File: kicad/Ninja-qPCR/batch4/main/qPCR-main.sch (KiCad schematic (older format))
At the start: 38 parts, among them J1 Raspberry_Pi_3A_Plus_wpi, J2 Conn_01x03_Male, J3 Conn_01x01_Male, J4 Conn_01x01_Male, J5 Conn_02x03_Odd_Even, J6 Conn_02x03_Odd_Even, J7 Conn_02x03_Odd_Even, Q1 Q_NMOS_GSD, Q2 Q_NMOS_GSD, Q3 Q_NMOS_GSD, Q4 Q_NMOS_GSD, Q5 Q_NMOS_GSD, Q6 Q_NMOS_GSD, SW1 TACTILE_4

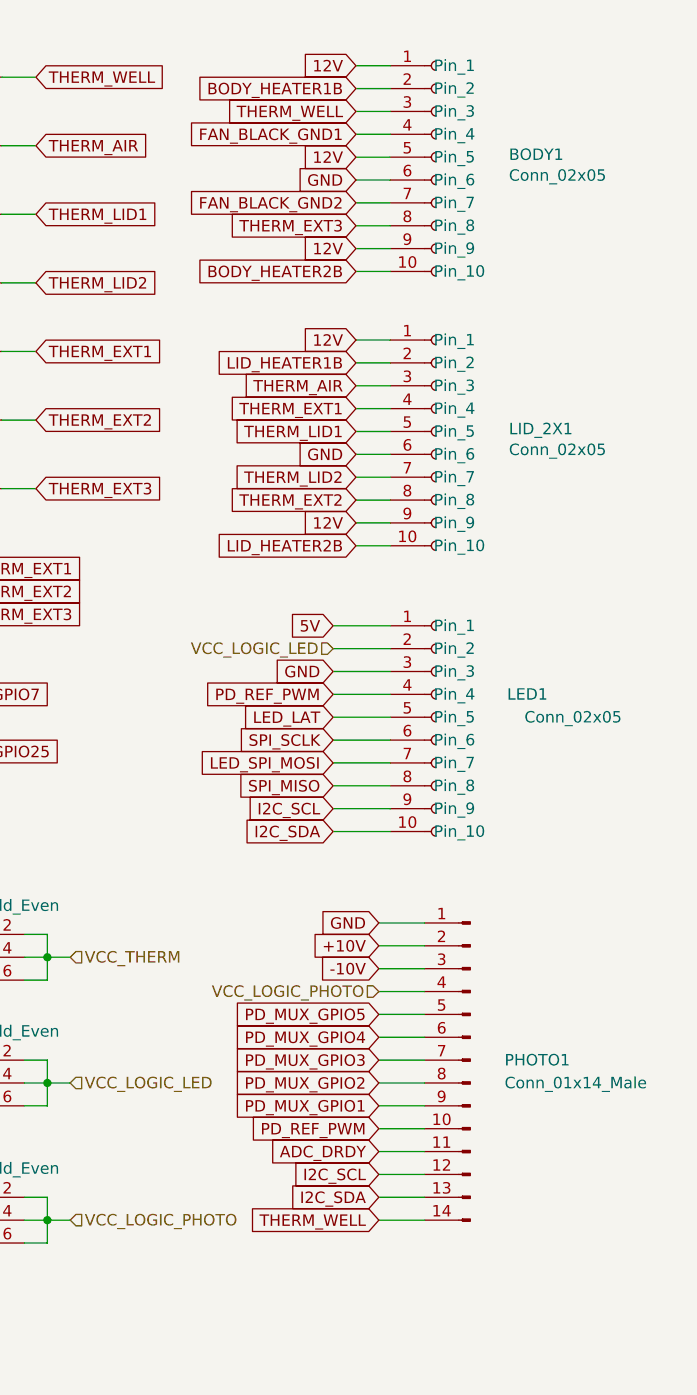
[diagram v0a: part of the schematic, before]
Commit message: add workflow
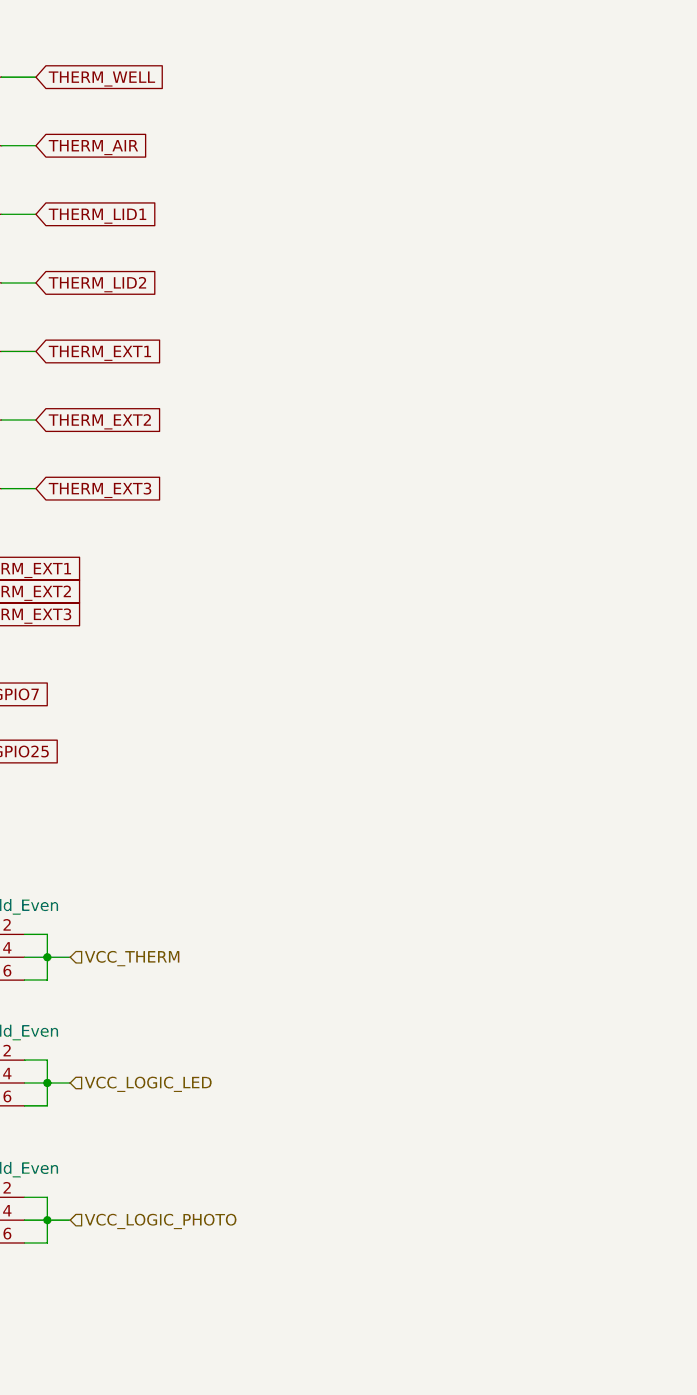
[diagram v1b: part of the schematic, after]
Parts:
- removed BODY1, LED1, LID_2X1: Conn_02x05, Ninja-qPCR:Con_2x05, symbol Ninja-qPCR:Conn_02x05
- removed PHOTO1: Conn_01x14_Male, Pin_Headers:Pin_Header_Straight_1x14_Pitch2.54mm, symbol Connector:Conn_01x14_Male
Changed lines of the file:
@@
 Wire Wire Line
 	2150 2950 2000 2950
-Text GLabel 9950 4700 0    50   Input ~ 0
-GND
-Wire Wire Line
-	9950 4700 10150 4700
-Wire Wire Line
-	10150 4800 9950 4800
-Wire Wire Line
-	9950 4900 10150 4900
-Wire Wire Line
-	10150 5000 9950 5000
-Wire Wire Line
-	9950 5100 10150 5100
-Wire Wire Line
-	10150 5200 9950 5200
-Wire Wire Line
-	9950 5300 10150 5300
-Wire Wire Line
-	10150 5400 9950 5400
-Wire Wire Line
-	9950 5500 10150 5500
-$Comp
-L Ninja-qPCR:Conn_02x05 LED1
-U 1 1 5F7E3B13
-P 10200 3400
-AR Path="/5F7E3B13" Ref="LED1"  Part="1"
-AR Path="/5F708CA1/5F7E3B13" Ref="LED?"  Part="1"
-F 0 "LED1" H 10600 3100 50  0000 C CNN
-F 1 "Conn_02x05" H 10800 3000 50  0000 C CNN
-F 2 "Ninja-qPCR:Con_2x05" H 10000 3500 50  0001 C CNN
-F 3 "" H 10000 3500 50  0001 C CNN
-	1    10200 3400
-	1    0    0    -1
-$EndComp
-Text GLabel 9750 3600 0    50   Input ~ 0
-GND
-Text GLabel 9750 3700 0    50   Input ~ 0
-PD_REF_PWM
-Text GLabel 9750 3800 0    50   Input ~ 0
-LED_LAT
-Text GLabel 9750 4000 0    50   Input ~ 0
-LED_SPI_MOSI
-Text GLabel 9750 4100 0    50   Input ~ 0
-SPI_MISO
-Text GLabel 9750 4200 0    50   Input ~ 0
-I2C_SCL
-Text GLabel 9750 4300 0    50   Input ~ 0
-I2C_SDA
-Wire Wire Line
-	9750 4300 10000 4300
-Wire Wire Line
-	9750 4200 10000 4200
-Wire Wire Line
-	9750 4100 10000 4100
-Wire Wire Line
-	9750 4000 10000 4000
-Wire Wire Line
-	9750 3900 10000 3900
-Wire Wire Line
-	9750 3800 10000 3800
-Wire Wire Line
-	9750 3700 10000 3700
-Wire Wire Line
-	9750 3600 10000 3600
-Wire Wire Line
-	9750 3500 10000 3500
-Wire Wire Line
-	9750 3400 10000 3400
-Text GLabel 9950 5100 0    50   Input ~ 0
-PD_MUX_GPIO5
-Text GLabel 9950 5200 0    50   Input ~ 0
-PD_MUX_GPIO4
-Text GLabel 9950 5400 0    50   Input ~ 0
-PD_MUX_GPIO2
-Text GLabel 9950 5300 0    50   Input ~ 0
-PD_MUX_GPIO3
-Text GLabel 9950 5500 0    50   Input ~ 0
-PD_MUX_GPIO1
-Text GLabel 9950 5600 0    50   Input ~ 0
-PD_REF_PWM
-Text GLabel 9950 5700 0    50   Input ~ 0
-ADC_DRDY
-Text GLabel 9950 5800 0    50   Input ~ 0
-I2C_SCL
-Text GLabel 9950 5900 0    50   Input ~ 0
-I2C_SDA
-Wire Wire Line
-	10150 5600 9950 5600
-Wire Wire Line
-	10150 5700 9950 5700
-Wire Wire Line
-	10150 5800 9950 5800
-Wire Wire Line
-	10150 5900 9950 5900
 Text GLabel 3700 3150 2    50   Input ~ 0
 THERM_AIR
-Text GLabel 9950 6000 0    50   Input ~ 0
-THERM_WELL
-Wire Wire Line
-	9950 6000 10150 6000
 Text GLabel 3700 3250 2    50   Input ~ 0
 THERM_LID1
 Text GLabel 3700 3350 2    50   Input ~ 0
 THERM_LID2
-$Comp
-L Ninja-qPCR:Conn_02x05 BODY?
-U 1 1 5F7E3B97
-P 10200 950
-AR Path="/5F58C19F/5F7E3B97" Ref="BODY?"  Part="1"
-AR Path="/5F7E3B97" Ref="BODY1"  Part="1"
-AR Path="/5F708CA1/5F7E3B97" Ref="BODY?"  Part="1"
-F 0 "BODY1" H 10519 561 50  0000 L CNN
-F 1 "Conn_02x05" H 10519 470 50  0000 L CNN
-F 2 "Ninja-qPCR:Con_2x05" H 10000 1050 50  0001 C CNN
-F 3 "" H 10000 1050 50  0001 C CNN
-	1    10200 950
-	1    0    0    -1
-$EndComp
-$Comp
-L Ninja-qPCR:Conn_02x05 LID_2X?
-U 1 1 5F7E3B9D
-P 10200 2150
-AR Path="/5F58C19F/5F7E3B9D" Ref="LID_2X?"  Part="1"
-AR Path="/5F7E3B9D" Ref="LID_2X1"  Part="1"
-AR Path="/5F708CA1/5F7E3B9D" Ref="LID_2X?"  Part="1"
-F 0 "LID_2X1" H 10519 1761 50  0000 L CNN
-F 1 "Conn_02x05" H 10519 1670 50  0000 L CNN
-F 2 "Ninja-qPCR:Con_2x05" H 10000 2250 50  0001 C CNN
-F 3 "" H 10000 2250 50  0001 C CNN
-	1    10200 2150
-	1    0    0    -1
-$EndComp
-Text GLabel 9850 1050 0    50   Input ~ 0
-BODY_HEATER1B
-Text GLabel 9850 1150 0    50   Input ~ 0
-THERM_WELL
-Text GLabel 9850 1250 0    50   Input ~ 0
-FAN_BLACK_GND1
-Text GLabel 9850 1450 0    50   Input ~ 0
-GND
-Text GLabel 9850 1550 0    50   Input ~ 0
-FAN_BLACK_GND2
-Text GLabel 9850 1650 0    50   Input ~ 0
-THERM_EXT3
-Text GLabel 9850 1850 0    50   Input ~ 0
-BODY_HEATER2B
-Wire Wire Line
-	10000 950  9850 950
-Wire Wire Line
-	9850 1050 10000 1050
-Wire Wire Line
-	10000 1150 9850 1150
-Wire Wire Line
-	9850 1250 10000 1250
-Wire Wire Line
-	10000 1350 9850 1350
-Wire Wire Line
-	9850 1450 10000 1450
-Wire Wire Line
-	10000 1550 9850 1550
-Wire Wire Line
-	9850 1650 10000 1650
-Wire Wire Line
-	10000 1750 9850 1750
-Wire Wire Line
-	9850 1850 10000 1850
-Text GLabel 9850 2250 0    50   Input ~ 0
-LID_HEATER1B
-Text GLabel 9850 3050 0    50   Input ~ 0
-LID_HEATER2B
-Text GLabel 9850 2350 0    50   Input ~ 0
-THERM_AIR
-Text GLabel 9850 2450 0    50   Input ~ 0
-THERM_EXT1
-Text GLabel 9850 2550 0    50   Input ~ 0
-THERM_LID1
-Text GLabel 9850 2650 0    50   Input ~ 0
-GND
-Text GLabel 9850 2750 0    50   Input ~ 0
-THERM_LID2
-Text GLabel 9850 2850 0    50   Input ~ 0
-THERM_EXT2
-Wire Wire Line
-	10000 2150 9850 2150
-Wire Wire Line
-	9850 2250 10000 2250
-Wire Wire Line
-	10000 2350 9850 2350
-Wire Wire Line
-	9850 2450 10000 2450
-Wire Wire Line
-	10000 2550 9850 2550
-Wire Wire Line
-	9850 2650 10000 2650
-Wire Wire Line
-	10000 2750 9850 2750
-Wire Wire Line
-	9850 2850 10000 2850
-Wire Wire Line
-	10000 2950 9850 2950
-Wire Wire Line
-	9850 3050 10000 3050
 Text GLabel 3700 2250 2    50   Input ~ 0
 SPI_SWITCH
@@
 Wire Wire Line
 	3650 1450 3700 1450
-$Comp
-L Connector:Conn_01x14_Male PHOTO1
-U 1 1 5F89D7B6
-P 10350 5300
-F 0 "PHOTO1" H 10200 5300 50  0000 R CNN
-F 1 "Conn_01x14_Male" H 10200 5200 50  0000 R CNN
-F 2 "Pin_Headers:Pin_Header_Straight_1x14_Pitch2.54mm" H 10350 5300 50  0001 C CNN
-F 3 "~" H 10350 5300 50  0001 C CNN
-	1    10350 5300
-	-1   0    0    -1
-$EndComp
 Wire Wire Line
 	8100 3350 7950 3350
@@
 	8200 3950 7950 3950
 NoConn ~ 2000 2250
-Text GLabel 9750 3900 0    50   Input ~ 0
-SPI_SCLK
 $Sheet
 S 5850 2650 850  250
@@
 Text HLabel 8600 6000 2    50   Input ~ 0
 VCC_LOGIC_PHOTO
-Text HLabel 9950 5000 0    50   Input ~ 0
-VCC_LOGIC_PHOTO
-Text HLabel 9750 3500 0    50   Input ~ 0
-VCC_LOGIC_LED
 $Comp
 L Connector_Generic:Conn_02x03_Odd_Even J6
@@
 Text GLabel 3700 1450 2    50   Input ~ 0
 5V
-Text GLabel 9750 3400 0    50   Input ~ 0
-5V
-Text GLabel 9950 4800 0    50   Input ~ 0
-+10V
-Text GLabel 9950 4900 0    50   Input ~ 0
--10V
 Text GLabel 7750 4750 0    50   Input ~ 0
 3V3_SENSE
@@
 Text GLabel 7750 6000 0    50   Input ~ 0
 3V3_REG
-Text GLabel 9850 950  0    50   Input ~ 0
-12V
-Text GLabel 9850 1350 0    50   Input ~ 0
-12V
-Text GLabel 9850 1750 0    50   Input ~ 0
-12V
-Text GLabel 9850 2150 0    50   Input ~ 0
-12V
-Text GLabel 9850 2950 0    50   Input ~ 0
-12V
 Wire Wire Line
 	4250 2900 4400 2900
